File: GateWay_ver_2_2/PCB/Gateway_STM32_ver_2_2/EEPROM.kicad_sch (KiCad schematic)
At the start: 8 parts, among them U13 CAT24C256

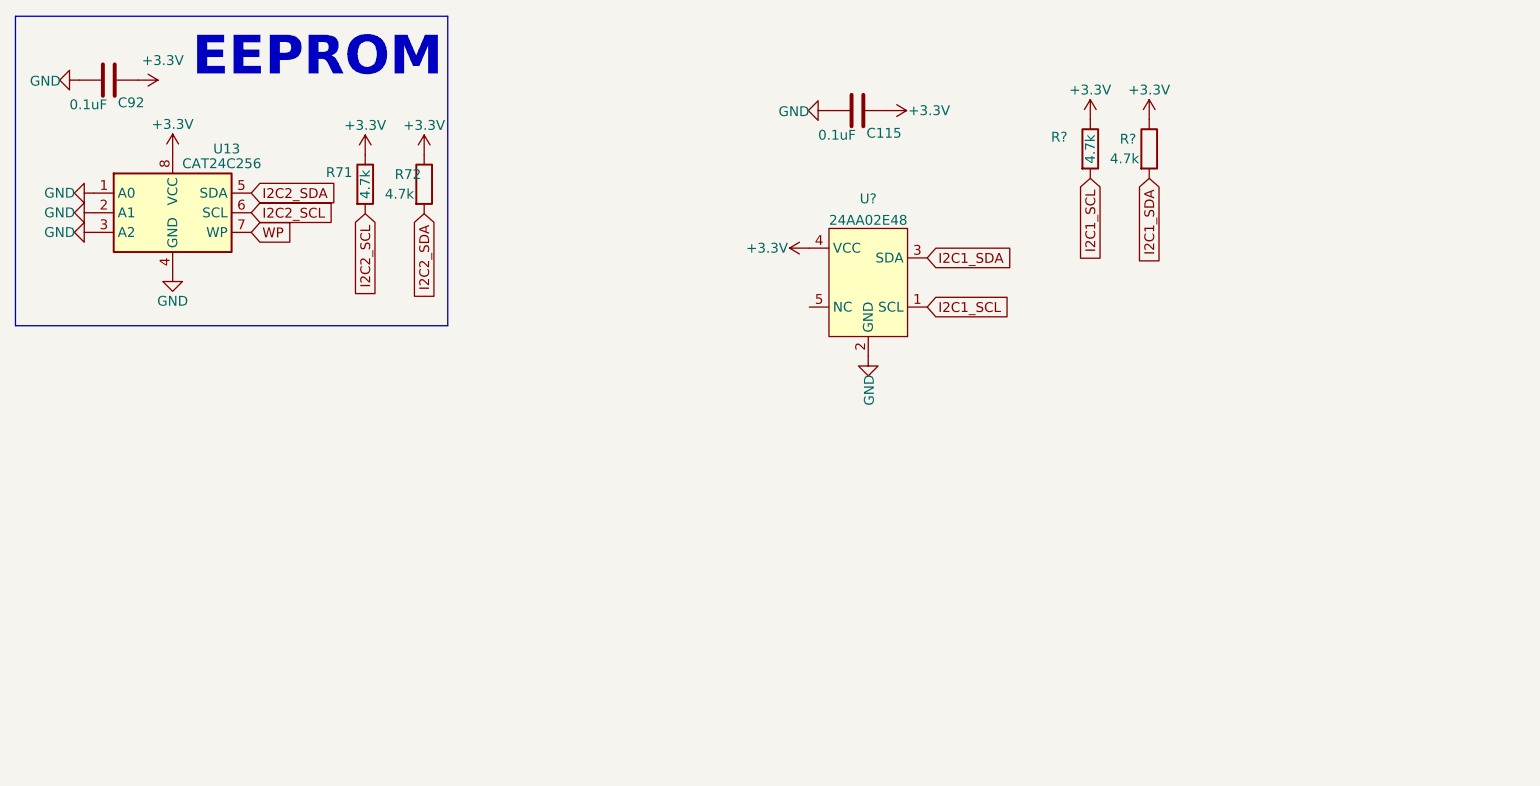
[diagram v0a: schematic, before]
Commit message: 1
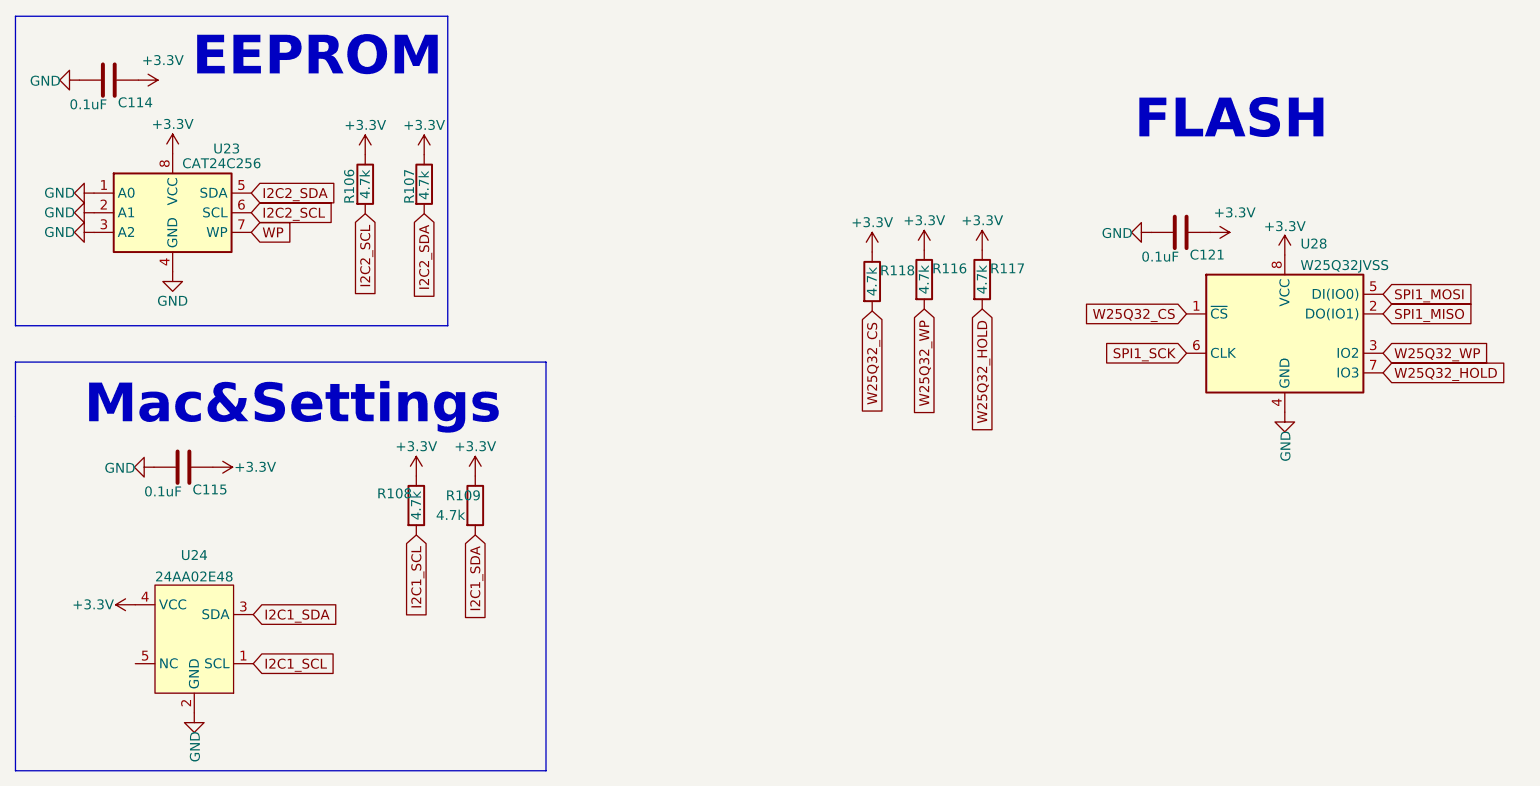
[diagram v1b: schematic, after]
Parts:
- added C121: 0.1uF, Capacitor_SMD:C_0603_1608Metric, symbol Device:C
- added R116, R117, R118: 4.7k, Resistor_SMD:R_0603_1608Metric, symbol Device:R
- added U28: W25Q32JVSS, Package_SO:SOIC-8_5.23x5.23mm_P1.27mm, symbol Memory_Flash:W25Q32JVSS
- gave numbers to parts that had none: 3
- renumbered C92 to C114, R71 to R106, R72 to R107, U13 to U23
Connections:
- net +3V3: now also C121.1, R116.1, R117.1, R118.1, U28.8 (VCC)
- net GND: now also C121.2, U28.4 (GND)
- new net SPI1_MISO: U28.2 (DO(IO1))
- new net SPI1_MOSI: U28.5 (DI(IO0))
- new net SPI1_SCK: U28.6 (CLK)
- new net W25Q32_CS: R118.2, U28.1 (~{CS})
- new net W25Q32_HOLD: R117.2, U28.7 (IO3)
- new net W25Q32_WP: R116.2, U28.3 (IO2)
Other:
- note added: "FLASH"
- note added: "Mac&Settings"
- moved on the sheet: C115, R108, R109, U24
